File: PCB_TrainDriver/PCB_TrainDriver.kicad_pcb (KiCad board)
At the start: 2 copper layers, 6.5 x 0.7 mm, 91 parts, among them CN1 XT90PW-M.G.Y, J1 Motor1_OUT, J2 Motor2_OUT, J3 aux_port1, J4 aux_port2, J5 aux_port3, Q1 BSC014N04LS, Q10 BSC014N04LS, Q11 BSC014N04LS, Q12 SS8050, Q13 SS8050, Q2 BSC014N04LS, Q3 BSC014N04LS, Q4 BSC014N04LS, Q5 BSC014N04LS, Q6 BSC014N04LS, Q7 BSC014N04LS, Q8 BSC014N04LS, Q9 BSC014N04LS, SW1 SW_Push, U1 DRV8701ERGER, U2 DRV8701ERGER, U3 ESP32-S3-WROOM-1, U4 TPS62932, U5 CH343P, U6 INA219AxDCN, U7 USBLC6-2P6, U9 LDL1117S33R

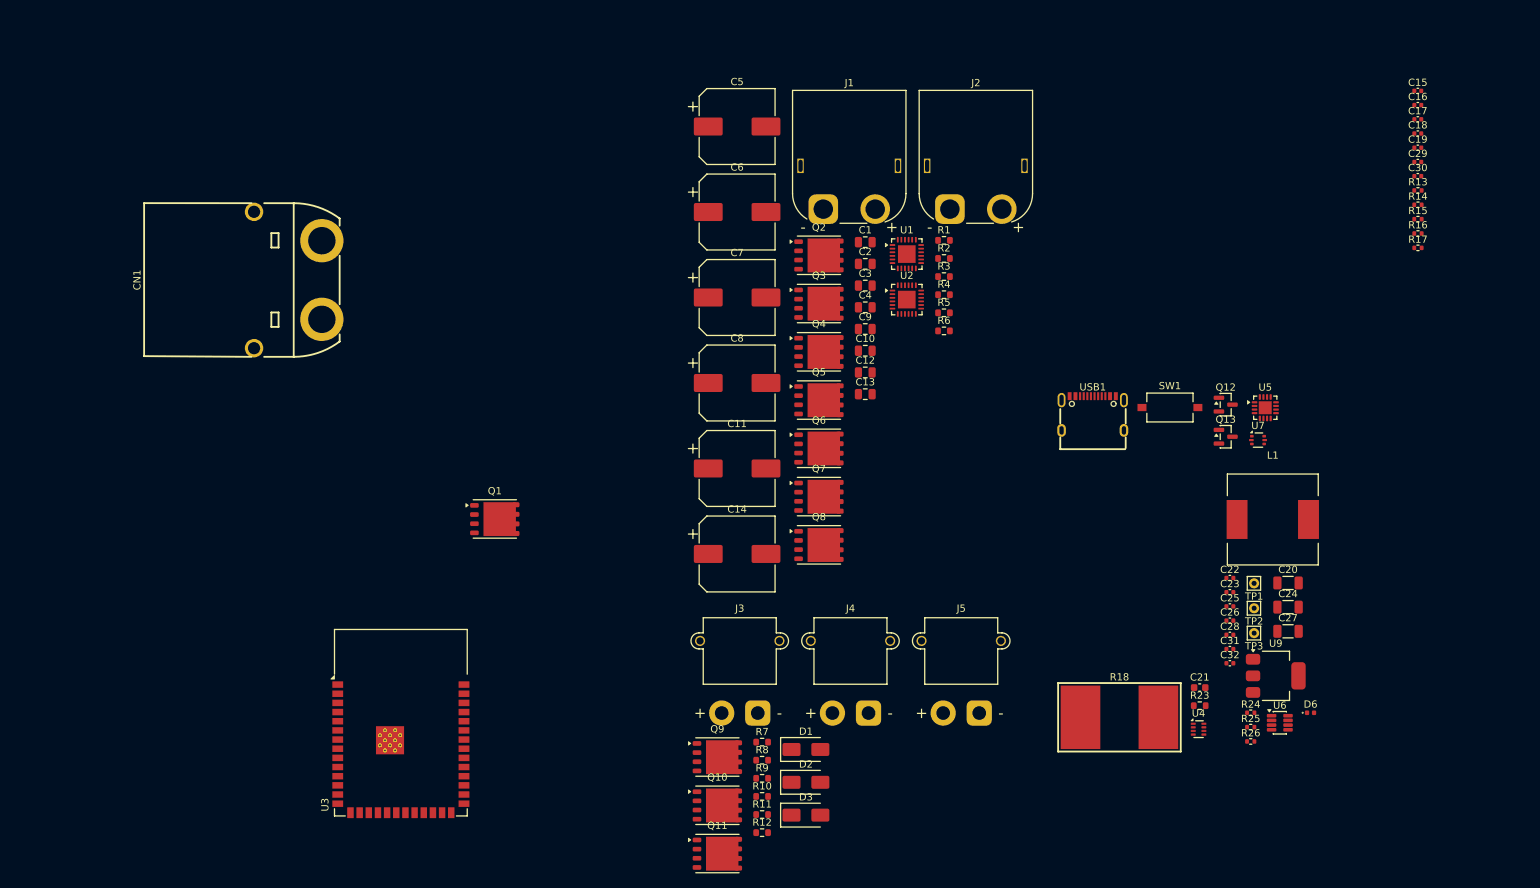
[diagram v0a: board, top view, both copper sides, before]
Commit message: PCB Almost Finished
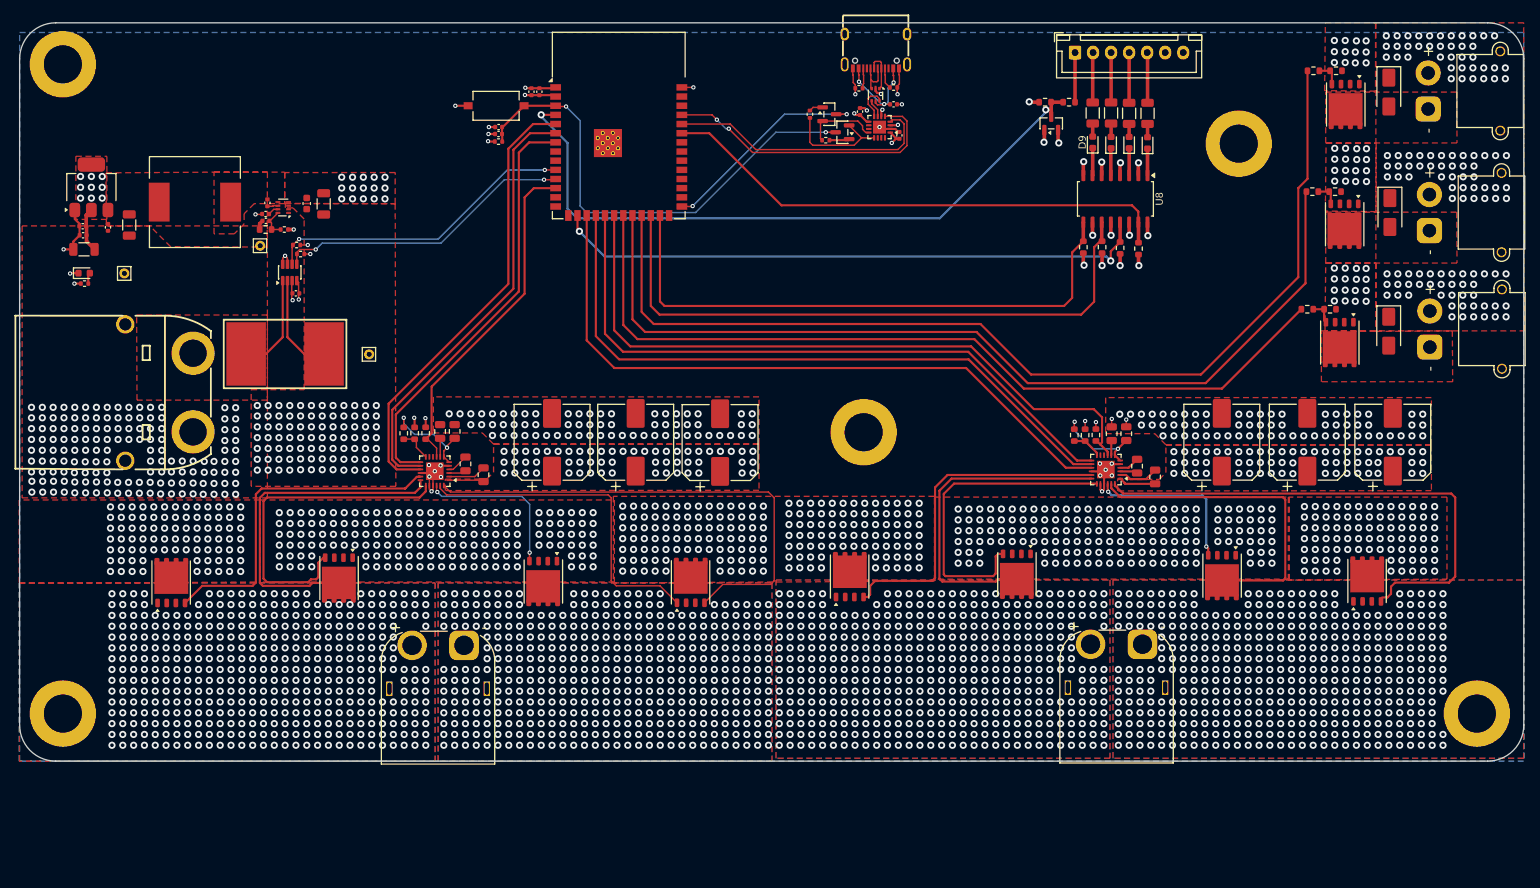
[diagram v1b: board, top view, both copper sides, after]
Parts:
- added D10: LED, LED_SMD:LED_0603_1608Metric, F.Cu at (200.3, 57.9)
- added D11: LED, LED_SMD:LED_0603_1608Metric, F.Cu at (202.8, 57.9)
- added D12: LED, LED_SMD:LED_0603_1608Metric, F.Cu at (205.3, 57.9)
- added D4: BAT54S, Package_TO_SOT_SMD:SOT-23, F.Cu at (192.0, 55.2)
- added D9: LED, LED_SMD:LED_0603_1608Metric, F.Cu at (197.8, 57.8)
- added H1: MountingHole, MountingHole:MountingHole_5.3mm_M5_DIN965_Pad, F.Cu at (55.0, 137.0)
- added H2: MountingHole, MountingHole:MountingHole_5.3mm_M5_DIN965_Pad, F.Cu at (251.0, 137.0)
- added H3: MountingHole, MountingHole:MountingHole_5.3mm_M5_DIN965_Pad, F.Cu at (55.0, 47.0)
- added H4: MountingHole, MountingHole:MountingHole_5.3mm_M5_DIN965_Pad, F.Cu at (166.0, 98.0)
- added H5: MountingHole, MountingHole:MountingHole_5.3mm_M5_DIN965_Pad, F.Cu at (218.0, 58.0)
- added J6: JoyStickConnector, Connector_JST:JST_XH_B7B-XH-A_1x07_P2.50mm_Vertical, F.Cu at (195.3, 45.4)
- added R19: 33k, Resistor_SMD:R_0603_1608Metric, F.Cu at (194.5, 52.2)
- added R20: 10k, Resistor_SMD:R_0603_1608Metric, F.Cu at (204.1, 72.5)
- added R21: 10k, Resistor_SMD:R_0603_1608Metric, F.Cu at (201.6, 72.5)
- added R22: 10k, Resistor_SMD:R_0603_1608Metric, F.Cu at (199.1, 72.3)
- added R27: 1k, Resistor_SMD:R_0402_1005Metric, F.Cu at (58.0, 77.4)
- added R28: 10k, Resistor_SMD:R_0603_1608Metric, F.Cu at (191.2, 52.2)
- added R29: 10k, Resistor_SMD:R_0603_1608Metric, F.Cu at (196.4, 72.3)
- added R30: 22k, Resistor_SMD:R_1206_3216Metric, F.Cu at (197.8, 53.8)
- added R31: 22k, Resistor_SMD:R_1206_3216Metric, F.Cu at (200.3, 53.8)
- added R32: 22k, Resistor_SMD:R_1206_3216Metric, F.Cu at (202.8, 53.8)
- added R33: 22k, Resistor_SMD:R_1206_3216Metric, F.Cu at (205.3, 53.8)
- added U8: TLP291-4, Package_SO:SOIC-16_4.55x10.3mm_P1.27mm, F.Cu at (200.9, 65.7)
- C15, C16, C17, C18, C21, C25, C28, C29, C32: value 0.1uF -> 0.1uF 50V
- C19: value 10uF -> 10uF 10V
- C20: value 10uF -> 10uF 50V
- C22: value 33nF -> 33nF 10V
- C23: value 18pF -> 18pF 25V
- C24: value 47uF -> 47uF 16V
- D6: footprint LED_SMD:LED_0402_1005Metric -> LED_SMD:LED_0603_1608Metric
- moved D6 180.6 mm to (58.0, 76.0)
- moved U9 177.6 mm to (59.0, 64.0), turned to 90 degrees
- moved C27 175.1 mm to (57.9, 72.7), turned to 180 degrees
- moved C24 169.1 mm to (64.2, 69.3), turned to 90 degrees
- moved C26 167.7 mm to (57.8, 70.7), turned to 180 degrees
- moved C25 167.5 mm to (57.8, 69.5), turned to 180 degrees
- moved C31 166.1 mm to (61.2, 69.6), turned to -90 degrees
- moved TP3 164.3 mm to (63.5, 76.0)
- moved L1 155.8 mm to (73.3, 66.1), turned to 180 degrees
- moved U6 150.8 mm to (86.5, 75.8), turned to 90 degrees
- moved R24 149.8 mm to (85.7, 69.9), turned to 180 degrees
- moved R25 148.2 mm to (87.4, 72.0), turned to 180 degrees
- moved R26 148.0 mm to (88.0, 73.3), turned to 180 degrees
- moved TP2 146.7 mm to (82.3, 72.2)
- moved C28 146.2 mm to (83.3, 66.2), turned to 90 degrees
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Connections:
- J1 pad 1: /H-Bridge_Driver/SH1_1 -> /H-Bridge_Driver/SH2_1
- J1 pad 2: /H-Bridge_Driver/SH2_1 -> /H-Bridge_Driver/SH1_1
- J2 pad 1: /H-Bridge_Driver/SH1_2 -> /H-Bridge_Driver/SH2_2
- J2 pad 2: /H-Bridge_Driver/SH2_2 -> /H-Bridge_Driver/SH1_2
- U1 pad 17: /H-Bridge_Driver/GL1_1 -> /H-Bridge_Driver/GH1_1
- U1 pad 19: /H-Bridge_Driver/GH1_1 -> /H-Bridge_Driver/GL1_1
- U2 pad 17: /H-Bridge_Driver/GL1_2 -> /H-Bridge_Driver/GH1_2
- U2 pad 19: /H-Bridge_Driver/GH1_2 -> /H-Bridge_Driver/GL1_2
- U3 pad 12: /H-Bridge_Driver/EN_2 -> /H-Bridge_Driver/nFAULT_1
- U3 pad 16: unconnected-(U3-IO46-Pad16) -> /MCU/BackwardIN_3.3V
- U3 pad 18: /H-Bridge_Driver/nSLEEP_2 -> /H-Bridge_Driver/EN_2
- U3 pad 19: /H-Bridge_Driver/nFAULT_2 -> /H-Bridge_Driver/nSLEEP_2
- U3 pad 20: /MCU/Pneumatic -> /H-Bridge_Driver/nFAULT_2
- U3 pad 21: /MCU/Horn -> /MCU/Lamp
- U3 pad 22: /MCU/Lamp -> /MCU/Horn
- U3 pad 23: unconnected-(U3-IO21-Pad23) -> /MCU/Pneumatic
- U3 pad 24: unconnected-(U3-IO47-Pad24) -> /MCU/HornIN_3.3V
- U3 pad 25: unconnected-(U3-IO48-Pad25) -> /MCU/LampIN_3.3V
- U3 pad 35: unconnected-(U3-IO42-Pad35) -> /MCU/ForwardIN_3.3V
- U3 pad 4: /H-Bridge_Driver/EN_1 -> /MCU/Speed_ControlIN_3.3V
- U3 pad 6: /H-Bridge_Driver/nSLEEP_1 -> /H-Bridge_Driver/EN_1
- U3 pad 7: /H-Bridge_Driver/nFAULT_1 -> /H-Bridge_Driver/nSLEEP_1
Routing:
- net /MCU/Pneumatic: track 0.00 -> 142.7 mm
- net /MCU/Horn: track 0.00 -> 129.8 mm
- net /MCU/Lamp: track 0.00 -> 117.4 mm
- net /H-Bridge_Driver/nFAULT_2: track 0.00 -> 95.1 mm
- net /H-Bridge_Driver/PH_2: track 0.00 -> 94.6 mm
- net /MCU/Speed_ControlIN_3.3V: track 0.00 -> 94.1 mm, vias 0 -> 2
- net /H-Bridge_Driver/EN_2: track 0.00 -> 92.8 mm
- net /H-Bridge_Driver/nSLEEP_2: track 0.00 -> 91.1 mm
- net /MCU/HornIN_3.3V: track 0.00 -> 86.9 mm
- net /MCU/BackwardIN_3.3V: track 0.00 -> 83.5 mm, vias 0 -> 2
- net /MCU/LampIN_3.3V: track 0.00 -> 80.9 mm
- net GND: track 0.00 -> 79.4 mm, vias 0 -> 696
- net /MCU/ForwardIN_3.3V: track 0.00 -> 72.1 mm
- net /H-Bridge_Driver/GH2_2: track 0.00 -> 70.9 mm
- net /H-Bridge_Driver/GH2_1: track 0.00 -> 68.9 mm
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- added copper zone on F.Cu, net +12V
- added copper zone on In2.Cu, net +12V
- added copper zone on F.Cu, net +3.3V
- added copper zone on In2.Cu, net +3.3V
- added copper zone on F.Cu, net +5V
- added copper zone on B.Cu, net /H-Bridge_Driver/SH1_1
- added copper zone on F.Cu, net /H-Bridge_Driver/SH1_1
- added copper zone on B.Cu, net /H-Bridge_Driver/SH1_2
- added copper zone on F.Cu, net /H-Bridge_Driver/SH1_2
- added copper zone on B.Cu, net /H-Bridge_Driver/SH2_1
- added copper zone on F.Cu, net /H-Bridge_Driver/SH2_1
- added copper zone on B.Cu, net /H-Bridge_Driver/SH2_2
- added copper zone on F.Cu, net /H-Bridge_Driver/SH2_2
- added copper zone on B.Cu, net GND
- added copper zone on F.Cu, net GND
- added copper zone on In1.Cu, net GND
- added copper zone on F.Cu, net Net-(D1-A)
- added copper zone on F.Cu, net Net-(D2-A)
- added copper zone on F.Cu, net Net-(D3-A)
- added copper zone on F.Cu, net Net-(U4-SW)
- added copper zone on F.Cu, net VCC
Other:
- board size 6.5 x 0.7 mm -> 208.5 x 102.3 mm
- copper layers 2 -> 4
- board text added: "Q1"
